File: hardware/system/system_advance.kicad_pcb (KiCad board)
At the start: 2 copper layers, 528.9 x 87.2 mm, 43 parts, among them J1 CART_SOCKET_28P, J2 EXTENSION PINS, SW1 POWER, SW2 RESET, SW3 A, SW4 B, SW5 UP, SW6 DN, SW7 LF, SW8 RT, U1 LIPO_CHARGER, U2 SPI_DISPLAY

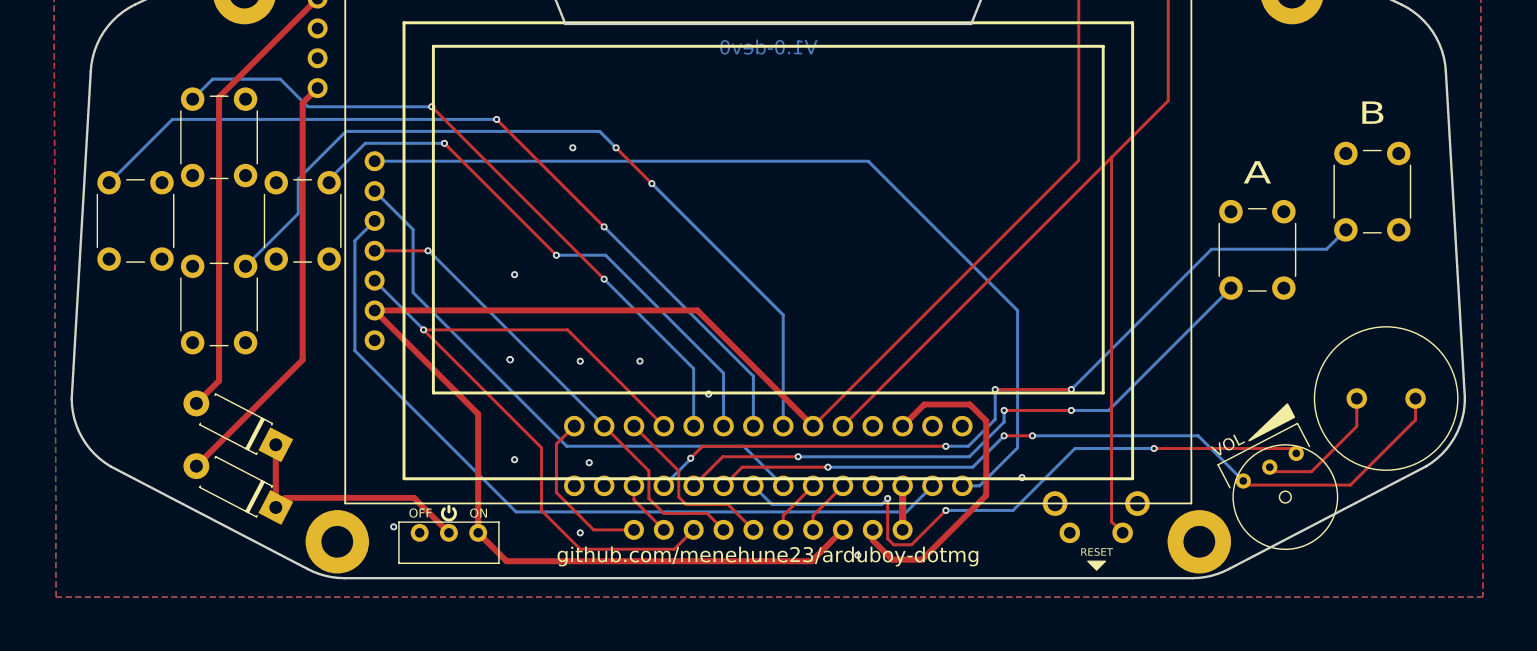
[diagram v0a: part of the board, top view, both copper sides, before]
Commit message: wip; board height adjust
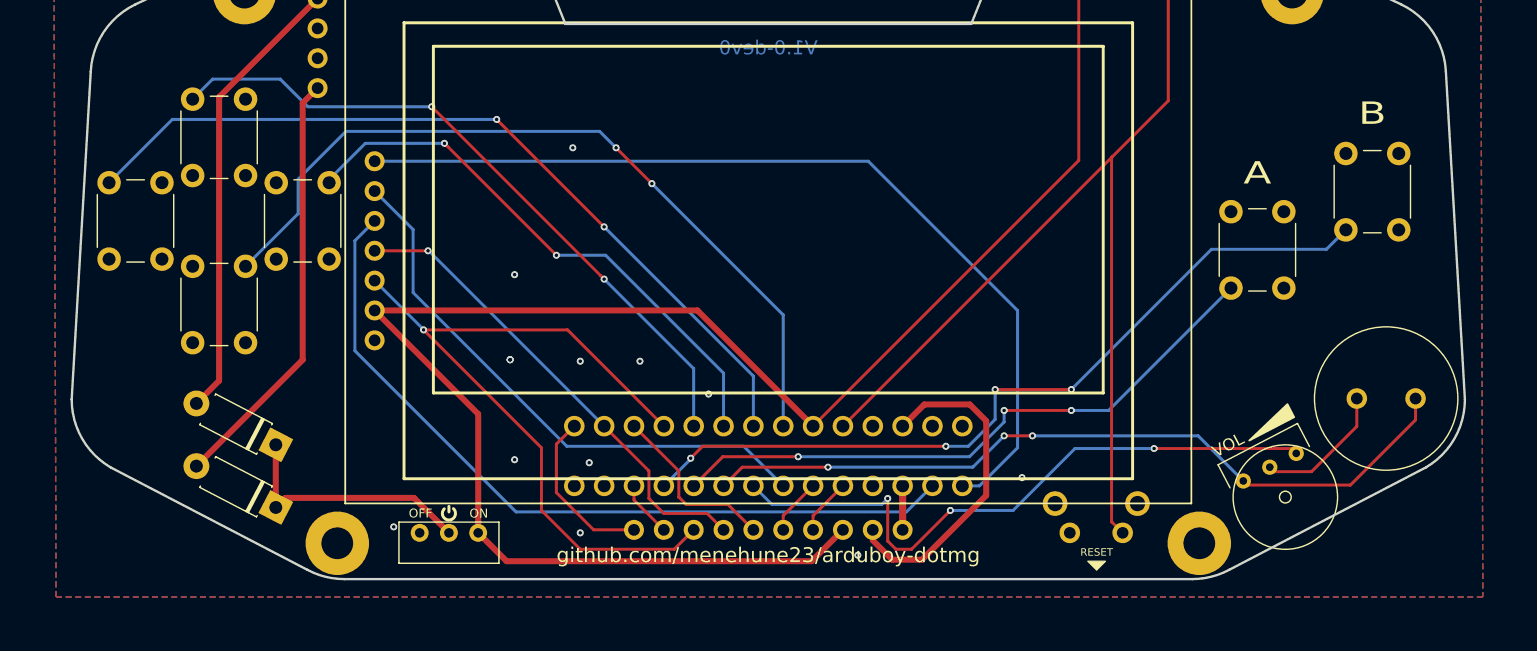
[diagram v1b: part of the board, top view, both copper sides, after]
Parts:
- moved HOLE 0.13 mm to (176.4, 119.9)
- moved HOLE 0.13 mm to (103.0, 119.9)
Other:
- outline, holes or cut-outs redrawn
- board text added: "W: 4.67” H: 2.2”"
- board text removed: "W: ???” H: ???”"
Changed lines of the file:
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@@
   )
   (module MountingHole:MountingHole_2.7mm_M2.5_Pad (layer B.Cu)
-    (at 103.0224 119.761 180)
+    (at 103.0224 119.888 180)
     (descr "Mounting Hole 2.7mm, M2.5")
     (tags "mounting hole 2.7mm m2.5")
@@
   )
   (module MountingHole:MountingHole_2.7mm_M2.5_Pad (layer F.Cu)
-    (at 176.3776 119.761)
+    (at 176.3776 119.888)
     (descr "Mounting Hole 2.7mm, M2.5")
     (tags "mounting hole 2.7mm m2.5")
@@
   (gr_arc (start 112.522 117.348) (end 112.903 116.9416) (angle 271.8476103) (layer F.SilkS) (width 0.254))
   (gr_line (start 112.522 116.7384) (end 112.522 117.221) (layer F.SilkS) (width 0.254))
-  (gr_line (start 83.730962 113.346323) (end 100.4824 122.068347) (layer Edge.Cuts) (width 0.2))
-  (gr_arc (start 87.122 107.569) (end 80.423 107.569) (angle -59.58891873) (layer Edge.Cuts) (width 0.2))
-  (gr_line (start 82.042 79.756) (end 80.423 107.569) (layer Edge.Cuts) (width 0.2))
+  (gr_line (start 83.727275 113.425423) (end 100.478713 122.147447) (layer Edge.Cuts) (width 0.2))
+  (gr_arc (start 87.118313 107.6481) (end 80.419313 107.6481) (angle -59.58891873) (layer Edge.Cuts) (width 0.2))
+  (gr_line (start 82.042 79.756) (end 80.419313 107.6481) (layer Edge.Cuts) (width 0.2))
   (gr_arc (start 88.741 80.07881) (end 82.042 79.756) (angle 61.67077339) (layer Edge.Cuts) (width 0.2))
   (gr_line (start 85.846224 74.028928) (end 99.563126 67.558209) (layer Edge.Cuts) (width 0.2))
@@
   (gr_line (start 118.11 67.056) (end 102.108 67.056) (layer Edge.Cuts) (width 0.2))
   (gr_line (start 161.29 67.056) (end 177.292 67.056) (layer Edge.Cuts) (width 0.2))
-  (gr_arc (start 103.635687 116.1579) (end 103.635687 122.8569) (angle 28.08040571) (layer Edge.Cuts) (width 0.2))
+  (gr_arc (start 103.632 116.237) (end 103.632 122.936) (angle 28.08040571) (layer Edge.Cuts) (width 0.2))
   (gr_line (start 193.553776 74.028928) (end 179.836874 67.558209) (layer Edge.Cuts) (width 0.2))
   (gr_arc (start 190.659 80.07881) (end 197.358 79.756) (angle -61.67077339) (layer Edge.Cuts) (width 0.2))
@@
     (effects (font (size 0.762 0.762) (thickness 0.1778)))
   )
-  (gr_text "W: ???”\nH: ???”" (at 67.818 94.488) (layer Cmts.User)
+  (gr_text "W: 4.67”\nH: 2.2”" (at 67.818 94.488) (layer Cmts.User)
     (effects (font (size 1 1) (thickness 0.15)) (justify left))
   )
@@
   (gr_poly (pts (xy 109.093 67.691) (xy 106.934 70.612) (xy 108.331 70.358)) (layer F.SilkS) (width 0.1))
   (gr_poly (pts (xy 164.338 112.724) (xy 164.338 77.724) (xy 194.338 77.724) (xy 194.338 112.724)) (layer Dwgs.User) (width 0.1))
-  (gr_arc (start 175.764313 116.1579) (end 175.764313 122.8569) (angle -28.08040571) (layer Edge.Cuts) (width 0.2))
+  (gr_arc (start 175.764313 116.237) (end 175.764313 122.936) (angle -28.08040571) (layer Edge.Cuts) (width 0.2))
   (gr_poly (pts (xy 167.64 122.174) (xy 168.402 121.412) (xy 166.878 121.412)) (layer F.SilkS) (width 0.1))
   (gr_text V1.0-dev0 (at 139.7 77.724) (layer B.Cu)
@@
     (effects (font (size 0.762 0.762) (thickness 0.1778)))
   )
-  (gr_line (start 197.358 79.756) (end 198.977 107.569) (layer Edge.Cuts) (width 0.2))
-  (gr_arc (start 192.278 107.569) (end 198.977 107.569) (angle 59.58891873) (layer Edge.Cuts) (width 0.2))
-  (gr_line (start 195.669038 113.346323) (end 178.9176 122.068347) (layer Edge.Cuts) (width 0.2))
-  (gr_line (start 175.764313 122.8569) (end 103.635687 122.8569) (layer Edge.Cuts) (width 0.2))
+  (gr_line (start 197.358 79.756) (end 198.977 107.6481) (layer Edge.Cuts) (width 0.2))
+  (gr_arc (start 192.278 107.6481) (end 198.977 107.6481) (angle 59.58891873) (layer Edge.Cuts) (width 0.2))
+  (gr_line (start 195.669038 113.425423) (end 178.9176 122.147447) (layer Edge.Cuts) (width 0.2))
+  (gr_line (start 175.764313 122.936) (end 103.635687 122.936) (layer Edge.Cuts) (width 0.2))
   (via (at 118.11 97.028) (size 0.6) (drill 0.3) (layers F.Cu B.Cu) (net 1))
   (via (at 128.778 104.394) (size 0.6) (drill 0.3) (layers F.Cu B.Cu) (net 1))
@@
   (segment (start 179.07 98.171) (end 168.656 108.585) (width 0.254) (layer B.Cu) (net 11))
   (via (at 149.86 116.078) (size 0.6) (drill 0.3) (layers F.Cu B.Cu) (net 12))
-  (via (at 154.813 117.094) (size 0.6) (drill 0.3) (layers F.Cu B.Cu) (net 12))
   (segment (start 140.016 116.586) (end 149.352 116.586) (width 0.254) (layer B.Cu) (net 12))
   (segment (start 149.352 116.586) (end 149.86 116.078) (width 0.254) (layer B.Cu) (net 12))
   (segment (start 138.43 115) (end 140.016 116.586) (width 0.254) (layer B.Cu) (net 12))
-  (segment (start 149.86 119.507) (end 150.368 120.015) (width 0.254) (layer F.Cu) (net 12))
-  (segment (start 151.892 120.015) (end 154.813 117.094) (width 0.254) (layer F.Cu) (net 12))
-  (segment (start 150.368 120.015) (end 151.892 120.015) (width 0.254) (layer F.Cu) (net 12))
-  (segment (start 149.86 116.078) (end 149.86 119.507) (width 0.254) (layer F.Cu) (net 12))
   (via (at 172.5295 111.8235) (size 0.6) (drill 0.3) (layers F.Cu B.Cu) (net 12))
-  (segment (start 165.7985 111.8235) (end 172.5295 111.8235) (width 0.254) (layer B.Cu) (net 12))
-  (segment (start 160.528 117.094) (end 165.7985 111.8235) (width 0.254) (layer B.Cu) (net 12))
-  (segment (start 154.813 117.094) (end 160.528 117.094) (width 0.254) (layer B.Cu) (net 12))
   (segment (start 184.210349 111.8235) (end 172.5295 111.8235) (width 0.254) (layer F.Cu) (net 12))
   (segment (start 184.625008 112.238159) (end 184.210349 111.8235) (width 0.254) (layer F.Cu) (net 12))
+  (segment (start 151.892 120.396) (end 155.194 117.094) (width 0.254) (layer F.Cu) (net 12))
+  (segment (start 149.86 119.6975) (end 150.5585 120.396) (width 0.254) (layer F.Cu) (net 12))
+  (segment (start 160.528 117.094) (end 155.194 117.094) (width 0.254) (layer B.Cu) (net 12))
+  (segment (start 150.5585 120.396) (end 151.892 120.396) (width 0.254) (layer F.Cu) (net 12))
+  (segment (start 149.86 116.078) (end 149.86 119.6975) (width 0.254) (layer F.Cu) (net 12))
+  (segment (start 172.5295 111.8235) (end 165.7985 111.8235) (width 0.254) (layer B.Cu) (net 12))
+  (segment (start 165.7985 111.8235) (end 160.528 117.094) (width 0.254) (layer B.Cu) (net 12))
+  (via (at 155.194 117.094) (size 0.6) (drill 0.3) (layers F.Cu B.Cu) (net 12))
   (segment (start 137.603 111.633) (end 140.97 115) (width 0.254) (layer B.Cu) (net 13))
   (segment (start 109.474 98.552) (end 122.555 111.633) (width 0.254) (layer B.Cu) (net 13))
